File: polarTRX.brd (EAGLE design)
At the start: 160 x 100 mm, 68 parts, among them Q1 NX-3215, U1 MAX4372F 50 Gain, U2 MCP1754S_SOT23, U3 PIC32MX250F128D, U4 LM94022, U5 LMP7702, X1 USB+SHIELD

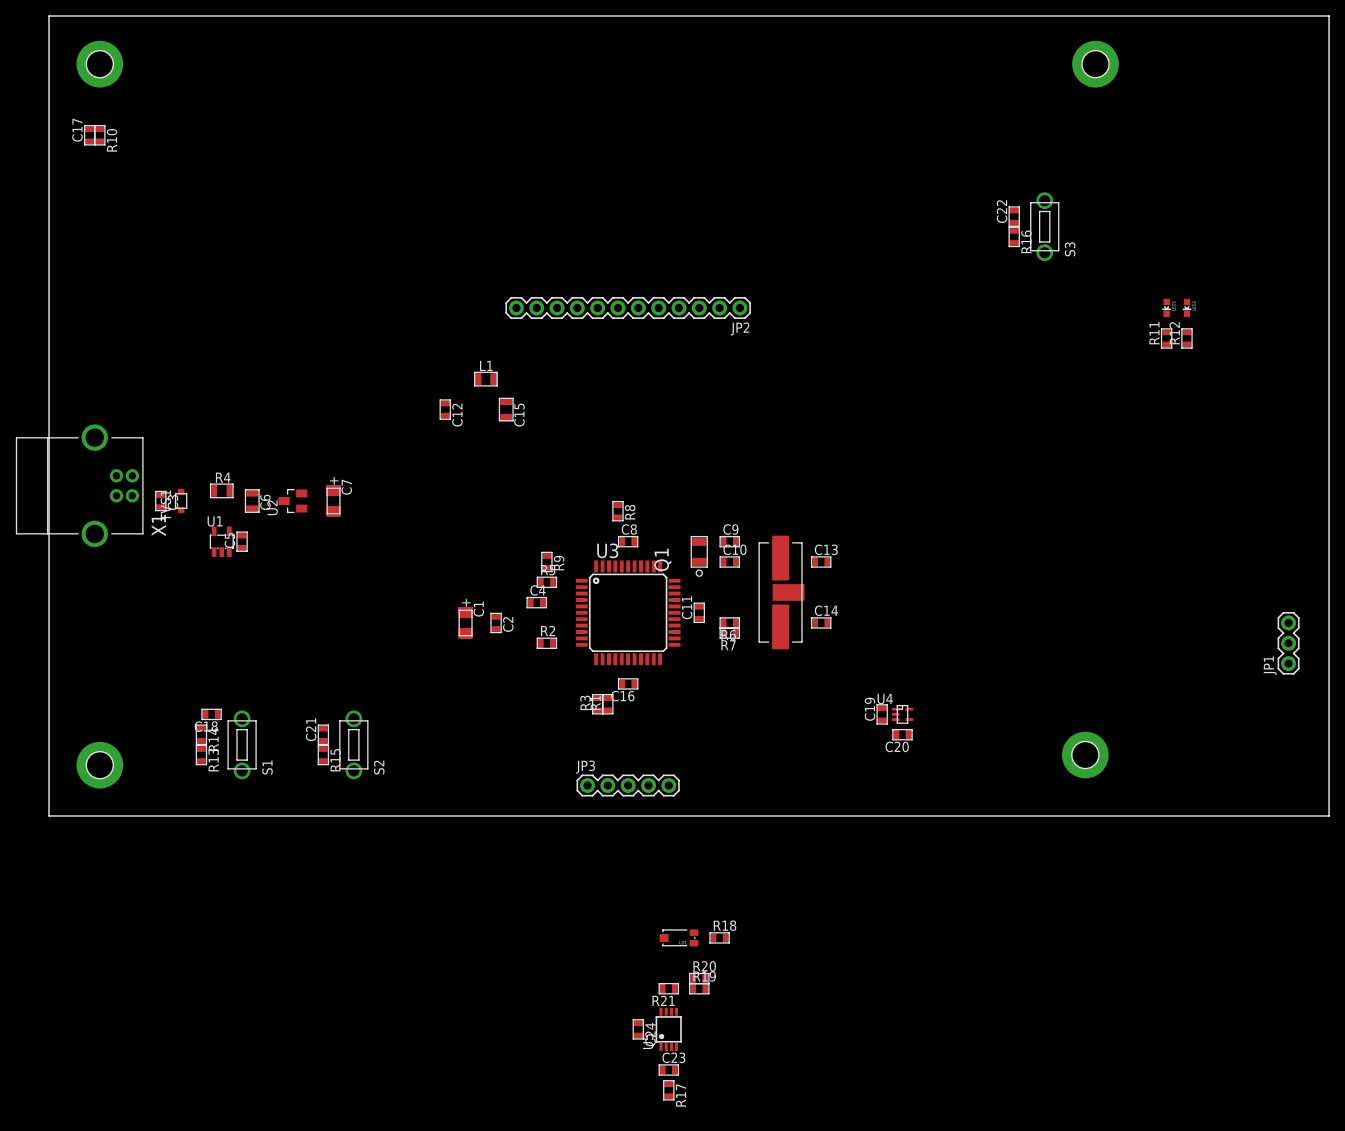
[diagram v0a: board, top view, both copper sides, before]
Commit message: board layout done
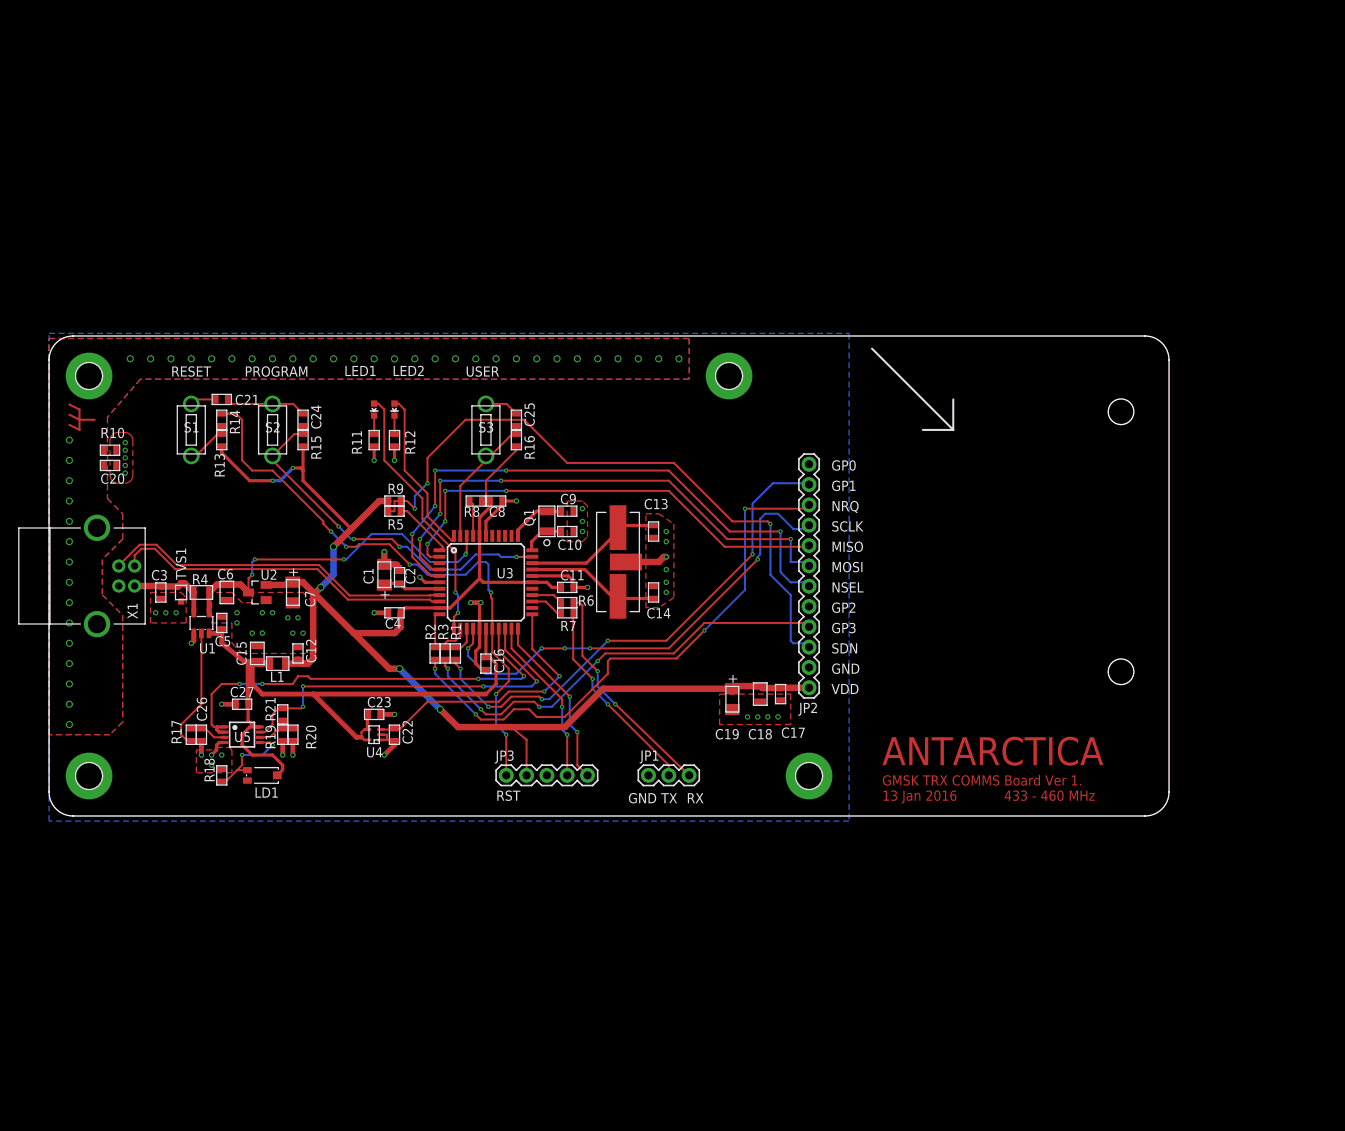
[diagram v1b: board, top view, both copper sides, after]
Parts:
- added C25, C26, C27: 0.1uF, polarinstruments:C0603(1608)
- C17: device yBrainDigital:C0603(1608) -> polarinstruments:C0603(1608)
- C18: value 0.1uF -> 10uF 0805; device polarinstruments:C0603(1608) -> polarinstruments:C0805(2012)
- C19: value 1100pF -> 10uF 16V; device polarinstruments:C0603(1608) -> berry:C1206(3216)-A
- C20: value 0.01uF -> 0.1uF; device polarinstruments:C0603(1608) -> yBrainDigital:C0603(1608)
- C22: value 0.1uF -> 1100pF
- C23: value 0.1uF -> 0.01uF
- moved C17 111.1 mm to (91.4, 15.2), turned to 270 degrees
- moved C20 104.6 mm to (7.62, 43.8)
- moved C22 101.0 mm to (43.2, 10.2), turned to 270 degrees
- moved LED2 99.9 mm to (43.2, 50.8)
- moved R12 99.9 mm to (43.2, 47.0)
- moved LED1 99.9 mm to (40.6, 50.8)
- moved R11 99.9 mm to (40.6, 47.0)
- moved C24 87.0 mm to (31.8, 49.5), turned to 90 degrees
- moved JP1 81.2 mm to (74.9, 5.08), turned to 0 degrees
- moved R17 74.4 mm to (17.8, 10.2)
- moved S3 74.3 mm to (54.6, 48.3)
- moved C18 68.6 mm to (88.9, 15.2), turned to 270 degrees
- moved R16 67.2 mm to (58.4, 47.0)
- moved U4 66.1 mm to (40.6, 10.2), turned to 90 degrees
- moved R18 65.5 mm to (21.6, 5.08), turned to 90 degrees
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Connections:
- net D+ renamed D_P
- net D- renamed D_N
- removed net AGND: C19.2, C20.2, C23.2, C24.2, C5.2, R18.2, R19.2, R20.2, U1.1, U3.16, U4.1, U4.2, U5.4
- removed net N$3: C6.1, R4.2, U1.4, U2.3
- new net N$7: C3.1, R4.1, TVS1.2, U1.5, X1.VBUS
- net +3.3V: now also C17.1, C18.1, C19.1
- net +3.3V_ANALOG: now also C23.1, C27.1; no longer C20.1, C24.1
- net +5V_USB: now also C6.1, R4.2, U1.4, U2.3; no longer C3.1, R4.1, TVS1.2, U1.5, X1.VBUS
- net DGND: now also C17.2, C19.2, C20.1, C23.2, C24.2, C25.2, C26.2, C27.2, C5.2, R18.2, R19.2, R20.2, U1.1, U3.16, U4.1, U4.2, U5.4; no longer C17.1
- net N$2: now also C21.1; no longer C18.1
- net N$21: now also C26.1; no longer C23.1
- net PRG: now also C24.1; no longer C21.1
- net STRUT_GND: now also C20.2; no longer C17.2
- net SW1: now also C25.1; no longer C22.1
- net TEMP_SENSE: now also C22.1; no longer C19.1
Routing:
- net +3.3V: track 0.00 -> 189.8 mm, vias 0 -> 6
- net +3.3V_ANALOG: track 0.00 -> 86.7 mm
- net RF_SDN: track 0.00 -> 80.5 mm, vias 0 -> 3
- net DGND: track 0.00 -> 76.3 mm, vias 0 -> 50
- net RESET: track 0.00 -> 74.8 mm, vias 0 -> 6
- net SS: track 0.00 -> 71.9 mm, vias 0 -> 5
- net RF_NIRQ: track 0.00 -> 69.7 mm, vias 0 -> 4
- net SDO: track 0.00 -> 65.7 mm, vias 0 -> 5
- net RF_GP1: track 0.00 -> 63.3 mm, vias 0 -> 5
- net SCK: track 0.00 -> 59.3 mm, vias 0 -> 5
- net SDI: track 0.00 -> 58.8 mm, vias 0 -> 4
- net AN0: track 0.00 -> 55.6 mm, vias 0 -> 4
- net RF_GP3: track 0.00 -> 54.8 mm, vias 0 -> 4
- net AN1: track 0.00 -> 47.7 mm, vias 0 -> 4
- net PRG: track 0.00 -> 45.6 mm, vias 0 -> 4
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- added copper zone on layer 1, net DGND
- added copper zone on layer 16, net DGND
- added copper zone on layer 1, net STRUT_GND
- added copper zone on layer 16, net STRUT_GND
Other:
- board size 160 x 100 mm -> 140 x 60 mm
- board text added: "13 Jan 2016"
- board text added: "433 - 460 MHz"
- board text added: "ANTARCTICA"
- board text added: "GMSK TRX COMMS Board Ver 1."
- board text added: "GND"
- board text added: "GP0"
- board text added: "GP1"
- board text added: "GP2"
- board text added: "GP3"
- board text added: "MISO"
- board text added: "MOSI"
- board text added: "NRQ"
- board text added: "NSEL"
- board text added: "PROGRAM"
- board text added: "RESET"
- board text added: "RST"
- board text added: "RX"
- board text added: "SCLK"
- board text added: "SDN"
- board text added: "TX"
- board text added: "USER"
- board text added: "VDD"
